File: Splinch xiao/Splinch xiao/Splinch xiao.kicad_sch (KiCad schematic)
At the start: 68 parts, among them SW2 Switch, U1 Seeeduino Xiao nRF52840

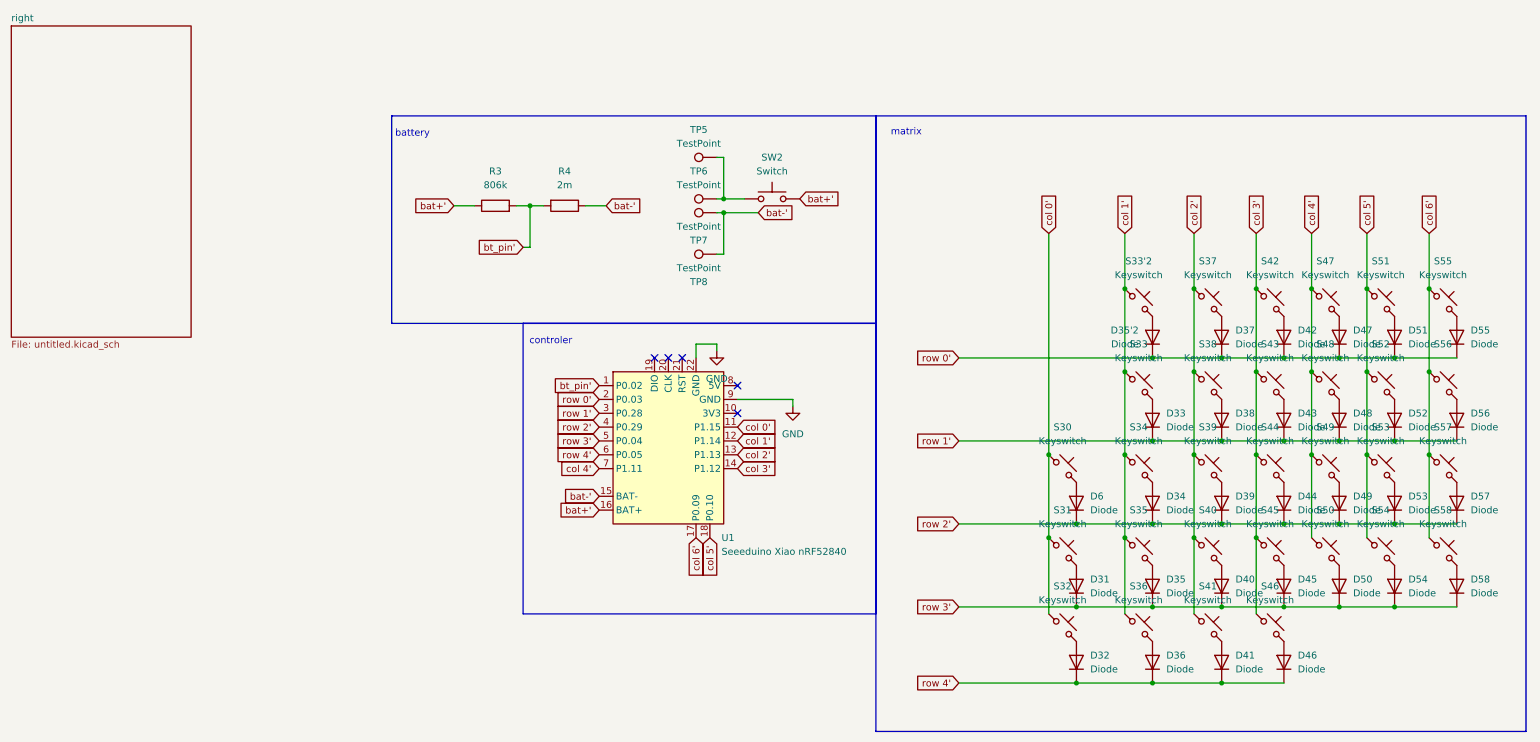
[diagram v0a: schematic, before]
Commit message: did some of the other galf
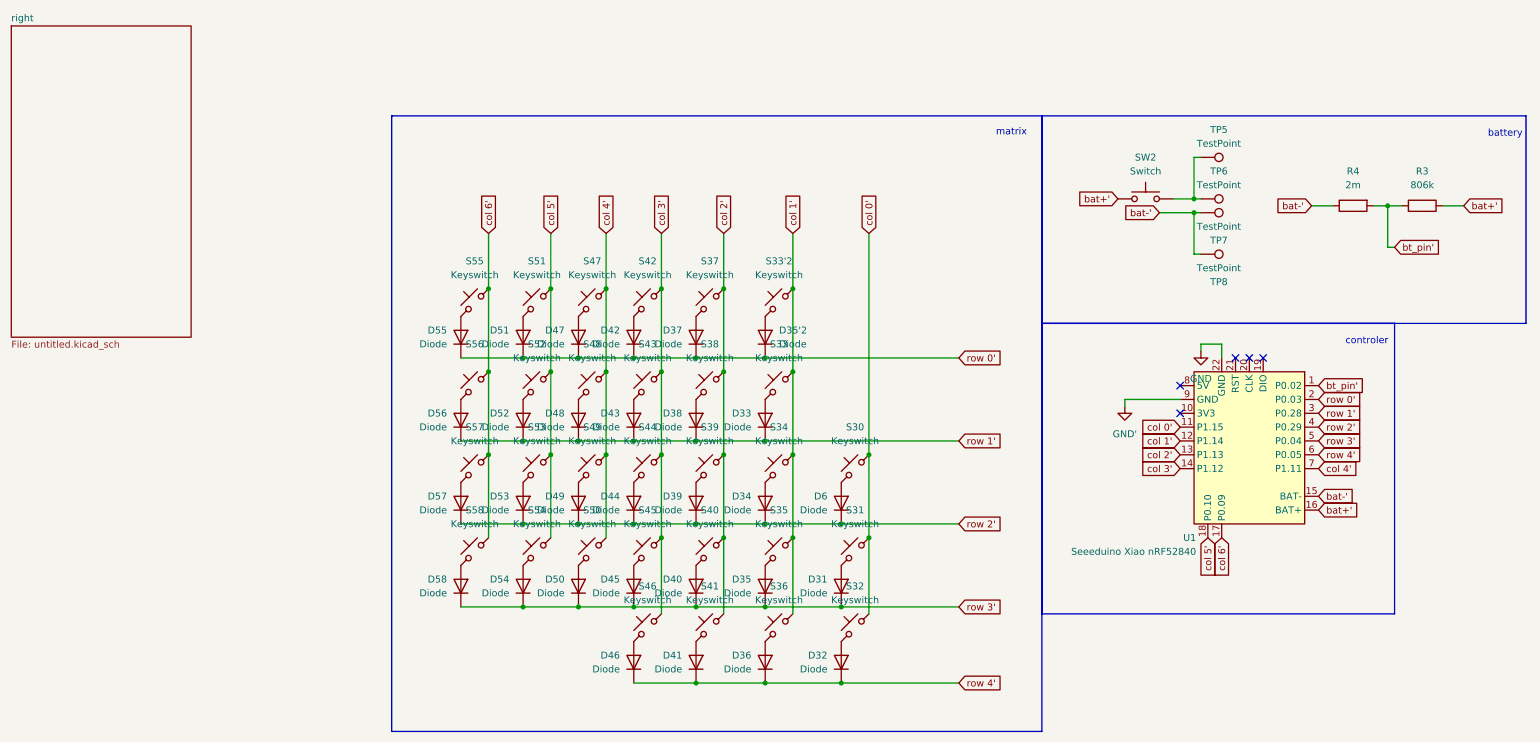
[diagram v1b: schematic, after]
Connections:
- net GND: no longer U1.9 (GND)
- new net GND': U1.9 (GND)
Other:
- moved on the sheet: D31, D32, D33, D34, D35, D35'2, D36, D37, D38, D39, D40, D41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
